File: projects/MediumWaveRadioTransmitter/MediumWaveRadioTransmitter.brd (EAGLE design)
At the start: 32.7 x 40.6 mm, 20 parts, among them P4 100k, Q1 400kH, T1 BC337, T2 BC337

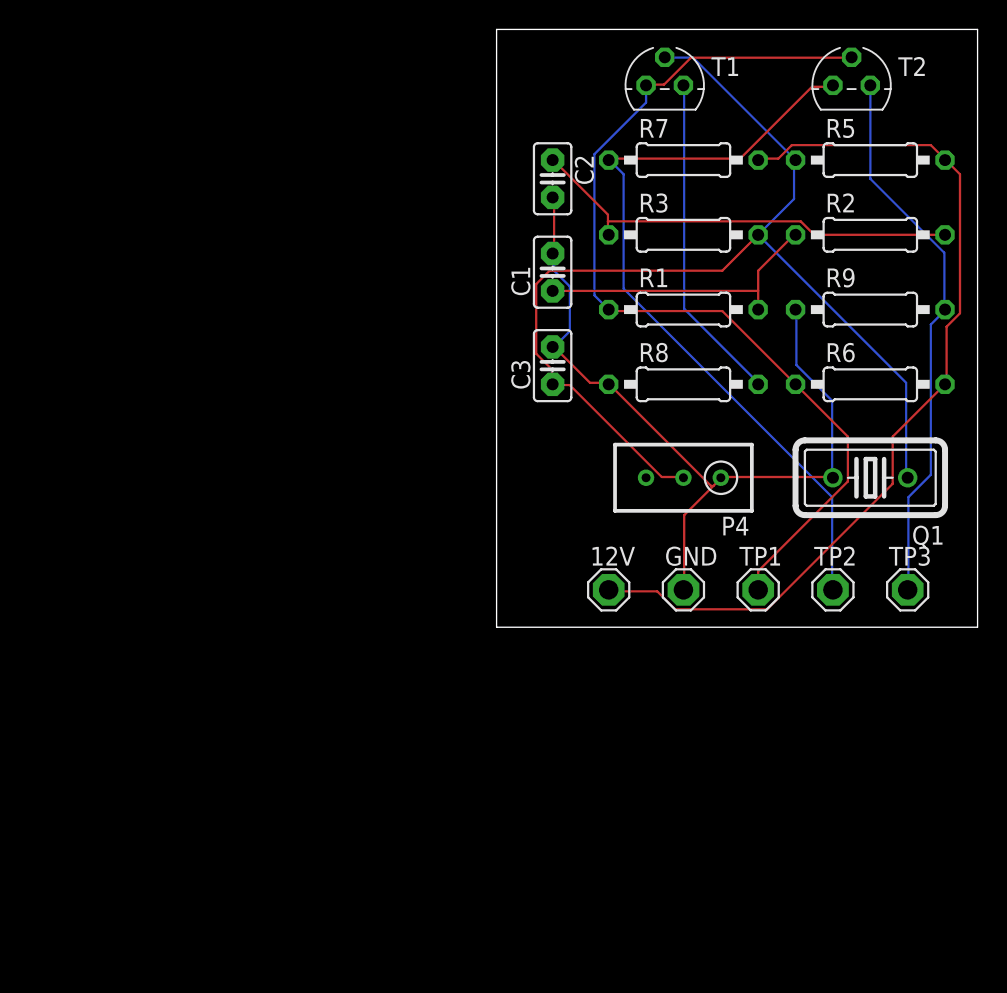
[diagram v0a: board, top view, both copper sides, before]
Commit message: fix: mwrt fixed a little bit
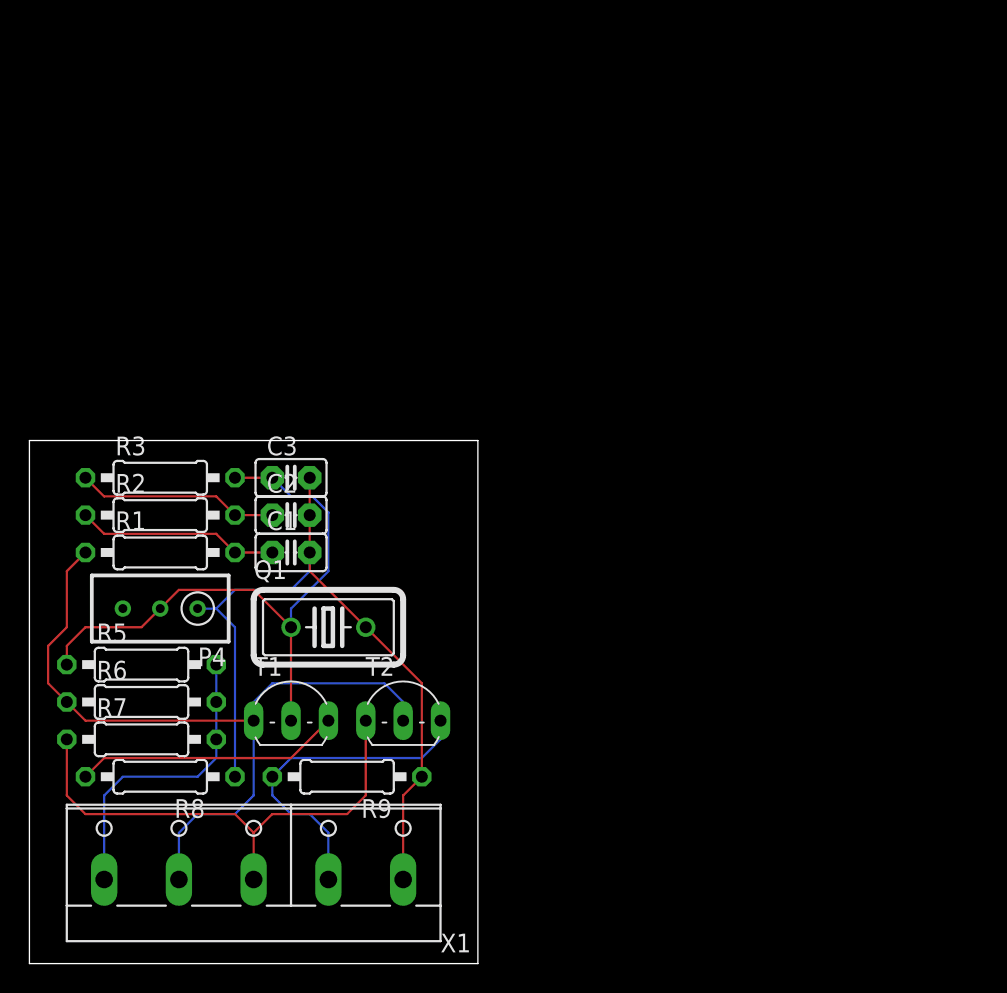
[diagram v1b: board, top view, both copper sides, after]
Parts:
- removed 12V, GND, TP1, TP2, TP3: SE13, solpad:SE13
- added X1: IN_OUT, con-wago-508:W237-5P
- T1, T2: device transistor:TO92 -> transistor:TO92-CBE
- moved R5 60.2 mm to (7.62, 20.3)
- moved R6 54.0 mm to (7.62, 17.8)
- moved R7 53.9 mm to (7.62, 15.2)
- moved T2 52.9 mm to (25.4, 16.5)
- moved R2 51.9 mm to (8.89, 30.5)
- moved T1 50.1 mm to (17.8, 16.5)
- moved R9 47.7 mm to (21.6, 12.7), turned to 180 degrees
- moved R8 44.5 mm to (8.89, 12.7), turned to 180 degrees
- moved R1 39.2 mm to (8.89, 27.9)
- moved R3 39.2 mm to (8.89, 33.0)
- moved Q1 38.2 mm to (20.3, 22.9), turned to 0 degrees
- moved P4 36.7 mm to (8.89, 24.1)
- moved C2 29.0 mm to (17.8, 30.5), turned to 0 degrees
- moved C1 26.1 mm to (17.8, 27.9), turned to 0 degrees
- moved C3 19.3 mm to (17.8, 33.0), turned to 0 degrees
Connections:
- removed net N$4: C1.2, C2.2, C3.2, GND.MP, P4.1, Q1.2, R8.1, R9.1
- new net GND: C1.2, C2.2, C3.2, P4.1, Q1.2, R8.1, R9.1, X1.5
- net N$10: now also T2.C, X1.3; no longer T2.3, TP2.MP
- net N$3: now also T1.B; no longer T1.2
- net N$5: now also T1.C, T2.B, X1.2; no longer T1.3, T2.2, TP1.MP
- net N$6: now also T1.E; no longer T1.1
- net N$7: now also X1.1; no longer 12V.MP
- net N$8: now also T2.E, X1.4; no longer T2.1, TP3.MP
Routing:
- net N$4: track 54.9 -> 0.00 mm
- net GND: track 0.00 -> 52.9 mm
- net N$7: track 61.3 -> 20.7 mm
- net N$3: track 73.9 -> 41.7 mm
- net N$10: track 52.9 -> 34.5 mm
- net N$2: track 30.0 -> 13.8 mm
- net N$8: track 37.4 -> 23.1 mm
- net N$5: track 64.6 -> 53.1 mm
- net N$1: track 20.2 -> 13.8 mm
- net N$6: track 22.4 -> 18.1 mm
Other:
- board size 32.7 x 40.6 mm -> 30.5 x 35.5 mm
